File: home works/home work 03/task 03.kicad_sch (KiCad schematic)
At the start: 0 parts

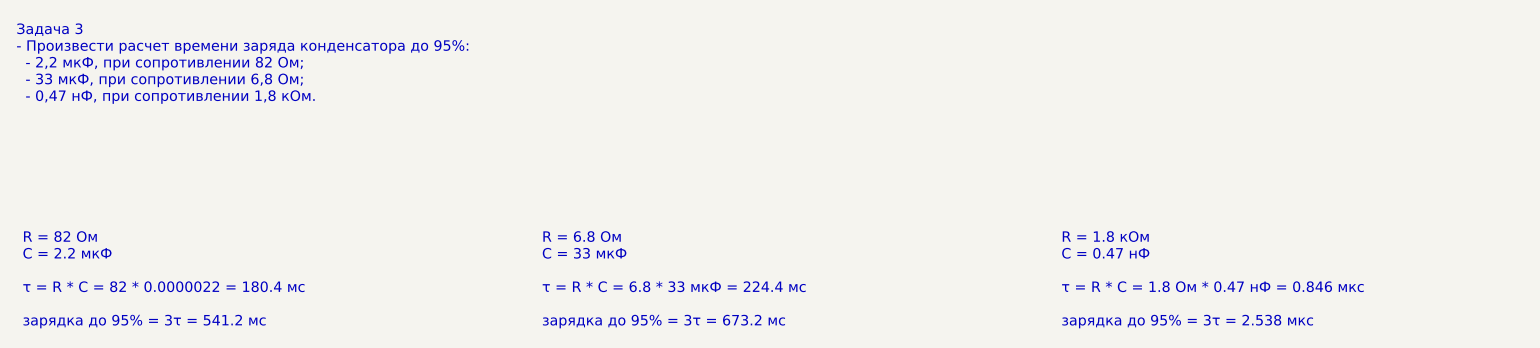
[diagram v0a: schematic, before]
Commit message: home works 3 and 4
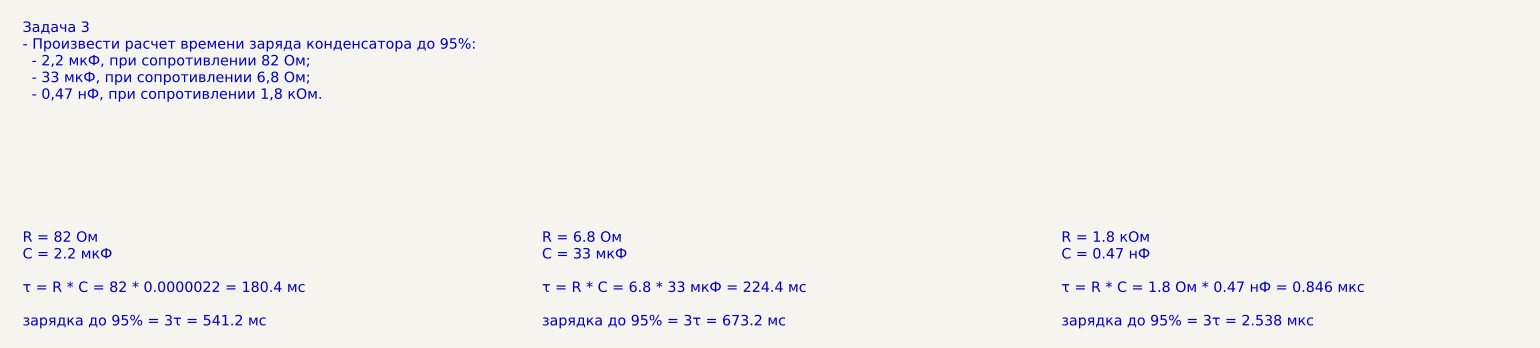
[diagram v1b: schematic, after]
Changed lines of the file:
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@@
 	(text "Задача 3 \n- Произвести расчет времени заряда конденсатора до 95%:\n  - 2,2 мкФ, при сопротивлении 82 Ом;\n  - 33 мкФ, при сопротивлении 6,8 Ом;\n  - 0,47 нФ, при сопротивлении 1,8 кОм."
 		(exclude_from_sim no)
-		(at 25.146 25.908 0)
+		(at 25.908 25.654 0)
 		(effects
 			(font
